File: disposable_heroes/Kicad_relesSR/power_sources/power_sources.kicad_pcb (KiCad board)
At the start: 4 copper layers, 96 x 90.6 mm, 18 parts, among them J1 V_{in}VB, J2 Transformer, J3 Power Sources, J4 5V_{VB}, U1 LM317_TO-220

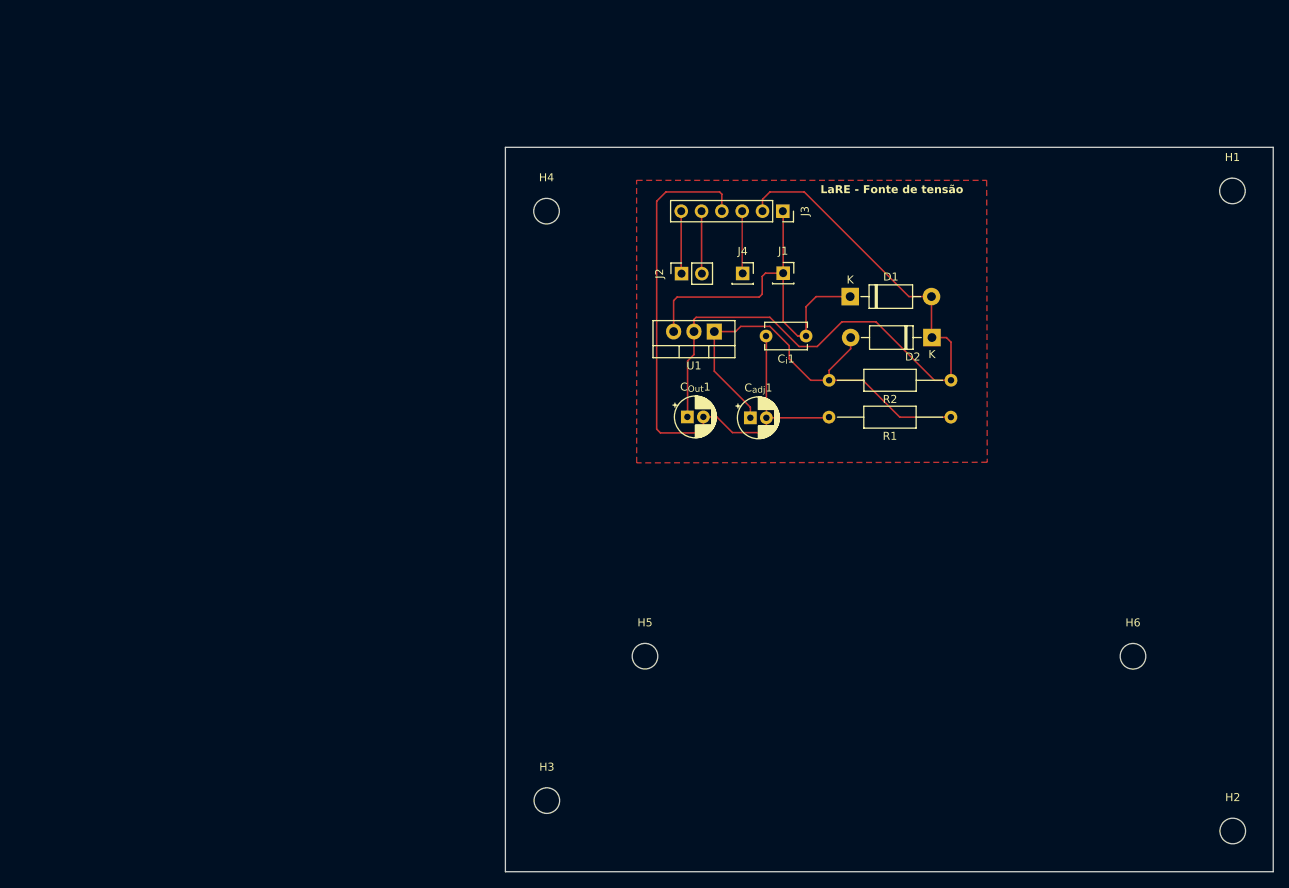
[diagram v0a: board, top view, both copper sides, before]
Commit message: update kicad files
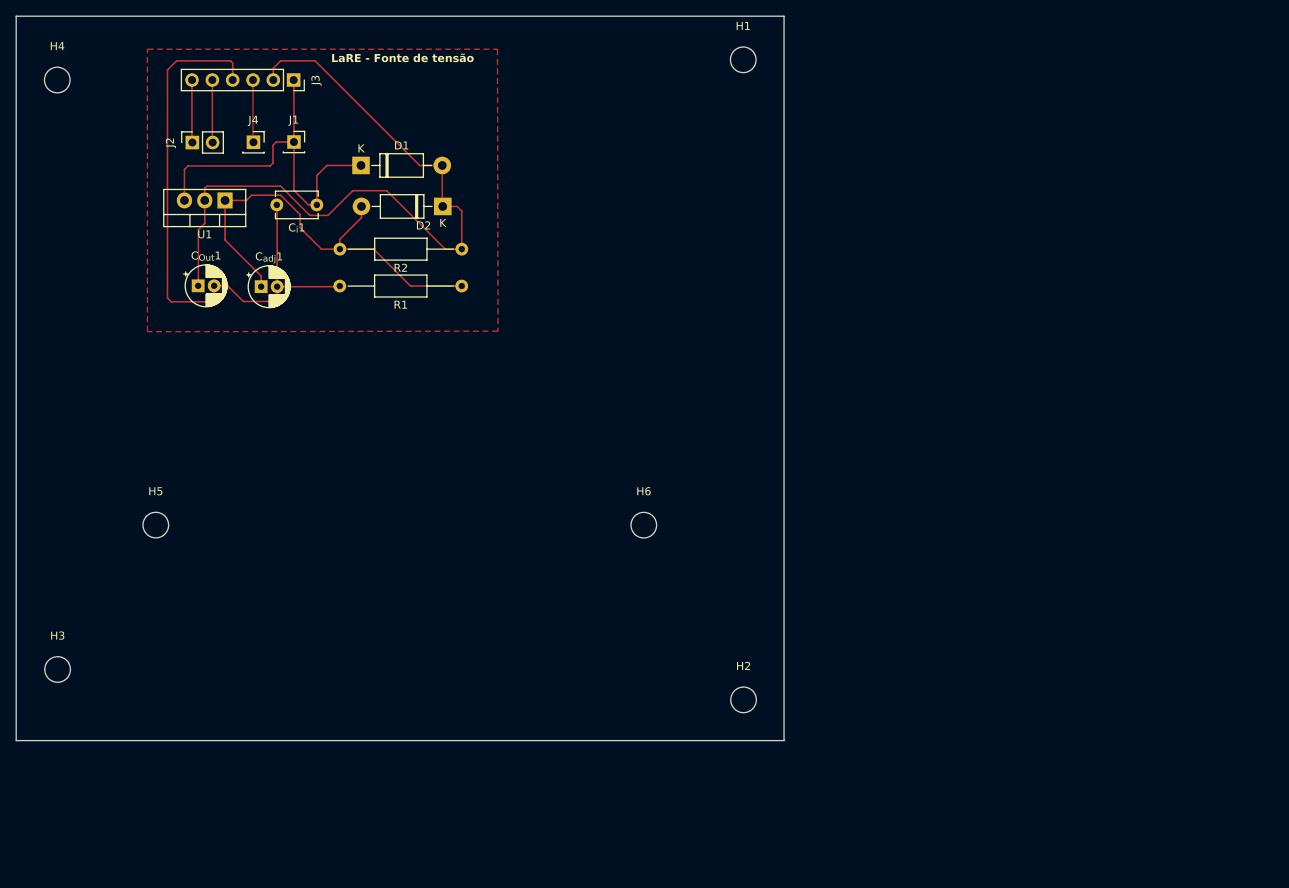
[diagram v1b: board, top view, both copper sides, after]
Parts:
- moved C_{Out}1 63.3 mm to (51.6, 57.2)
- moved C_{adj}1 63.3 mm to (59.5, 57.3)
- moved C_{i}1 63.3 mm to (66.5, 47.1)
- moved H5 63.3 mm to (46.3, 87.1)
- moved R1 63.3 mm to (84.6, 57.2)
- moved H4 63.3 mm to (34.0, 31.5)
- moved J1 63.3 mm to (63.6, 39.2)
- moved J2 63.3 mm to (50.9, 39.3)
- moved J4 63.3 mm to (58.5, 39.2)
- moved D1 63.3 mm to (72.0, 42.1)
- moved D2 63.3 mm to (82.2, 47.3)
- moved H1 63.3 mm to (119.8, 28.9)
- moved H2 63.3 mm to (119.8, 109.0)
- moved H3 63.3 mm to (34.1, 105.2)
- moved H6 63.3 mm to (107.3, 87.1)
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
